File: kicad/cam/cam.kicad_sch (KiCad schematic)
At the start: 4 parts, among them SW1 L101011_SPST, U1 S13V10FS, U2 ESP32-CAM

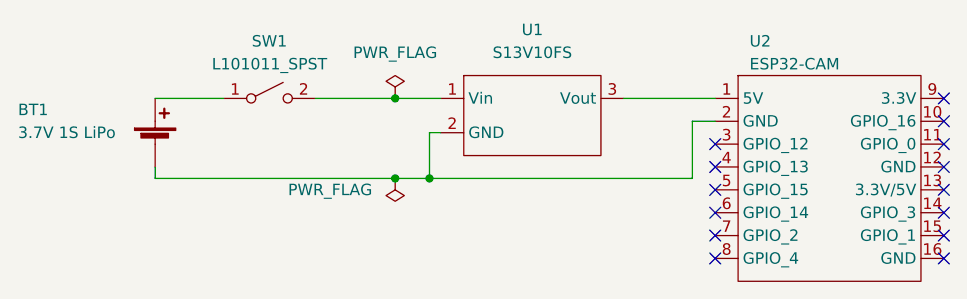
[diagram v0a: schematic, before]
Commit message: Cape 1.3, Main 1.7
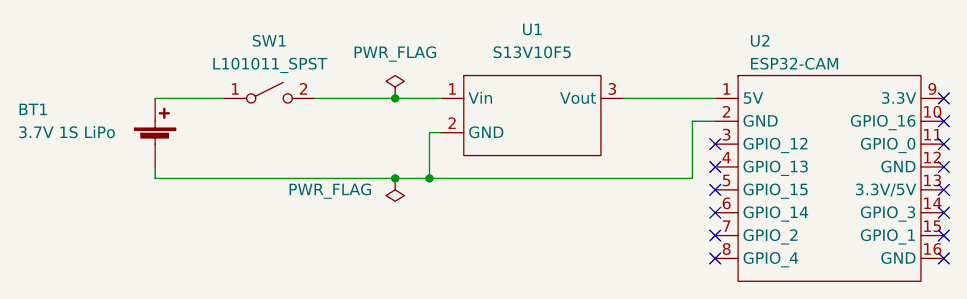
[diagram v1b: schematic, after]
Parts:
- U1: value S13V10FS -> S13V10F5
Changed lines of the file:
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@@
     (in_bom yes) (on_board yes) (fields_autoplaced)
     (property "Reference" "U1" (id 0) (at 80.01 21.59 0))
-    (property "Value" "S13V10FS" (id 1) (at 80.01 24.13 0))
+    (property "Value" "S13V10F5" (id 1) (at 80.01 24.13 0))
     (property "Footprint" "" (id 2) (at 87.63 26.67 0)
       (effects (font (size 1.27 1.27)) hide)
@@
     )
     (path "/70068c15-41a7-4281-88d5-2d9751a9bcef"
-      (reference "U1") (unit 1) (value "S13V10FS") (footprint "")
+      (reference "U1") (unit 1) (value "S13V10F5") (footprint "")
     )
     (path "/8be02d02-d42c-4113-9745-fb4efcc193ff"

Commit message: Updated all schematics
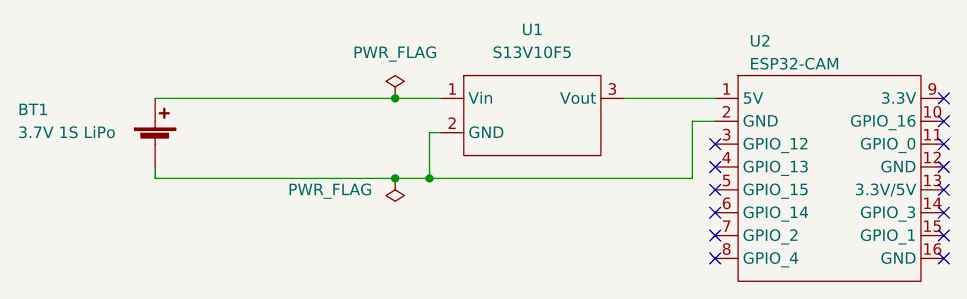
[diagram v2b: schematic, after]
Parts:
- removed SW1: L101011_SPST, symbol Switch:SW_SPST
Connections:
- net at U1.1 (Vin): now also BT1.1 (+)
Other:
- company: (none) -> Peter Costescu
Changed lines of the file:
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@@
     (title "Payload Camera Subsystem")
     (date "2022-12-29")
-    (rev "1.2")
+    (rev "1.3")
+    (company "Peter Costescu")
   )
   (junction (at 68.58 38.1) (diameter 0) (color 0 0 0 0)
@@
     (stroke (width 0) (type default) (color 0 0 0 0))
   )
-  (wire (pts (xy 55.88 29.21) (xy 64.77 29.21))
-    (stroke (width 0) (type default) (color 0 0 0 0))
-  )
-  (wire (pts (xy 38.1 29.21) (xy 45.72 29.21))
+  (wire (pts (xy 38.1 29.21) (xy 64.77 29.21))
     (stroke (width 0) (type default) (color 0 0 0 0))
   )
@@
     (stroke (width 0) (type default) (color 0 0 0 0))
   )
-  (image (at 68.58 63.5)
+  (image (at 86.36 63.5)
     (data
       iVBORw0KGgoAAAANSUhEUgAAAbIAAACKCAYAAADPLc9oAAAABHNCSVQICAgIfAhkiAAAAAlwSFlz
@@
     (pin "9")
   )
-  (symbol (lib_id "Switch:SW_SPST") (at 50.8 29.21 0) (unit 1)
-    (in_bom yes) (on_board yes) (fields_autoplaced)
-    (property "Reference" "SW1" (id 0) (at 50.8 22.86 0))
-    (property "Value" "L101011_SPST" (id 1) (at 50.8 25.4 0))
-    (property "Footprint" "" (id 2) (at 50.8 29.21 0)
-      (effects (font (size 1.27 1.27)) hide)
-    )
-    (property "Datasheet" "~" (id 3) (at 50.8 29.21 0)
-      (effects (font (size 1.27 1.27)) hide)
-    )
-    (pin "1")
-    (pin "2")
-  )
   (sheet_instances
     (path "/" (page "1"))
@@
       (reference "BT1") (unit 1) (value "3.7V 1S LiPo") (footprint "")
     )
-    (path "/d1891484-f2a6-457e-924d-ce3e4f9d53ae"
-      (reference "SW1") (unit 1) (value "L101011_SPST") (footprint "")
-    )
     (path "/70068c15-41a7-4281-88d5-2d9751a9bcef"
